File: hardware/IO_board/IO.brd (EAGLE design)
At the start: 167.9 x 122.5 mm, 52 parts, among them IC1 MAX232, IC4 74HCT139N, IC5 74AC06N, IC7 MAX232, J1 DIN5, X2 CRYSTALS-NOGND-CFPX-217

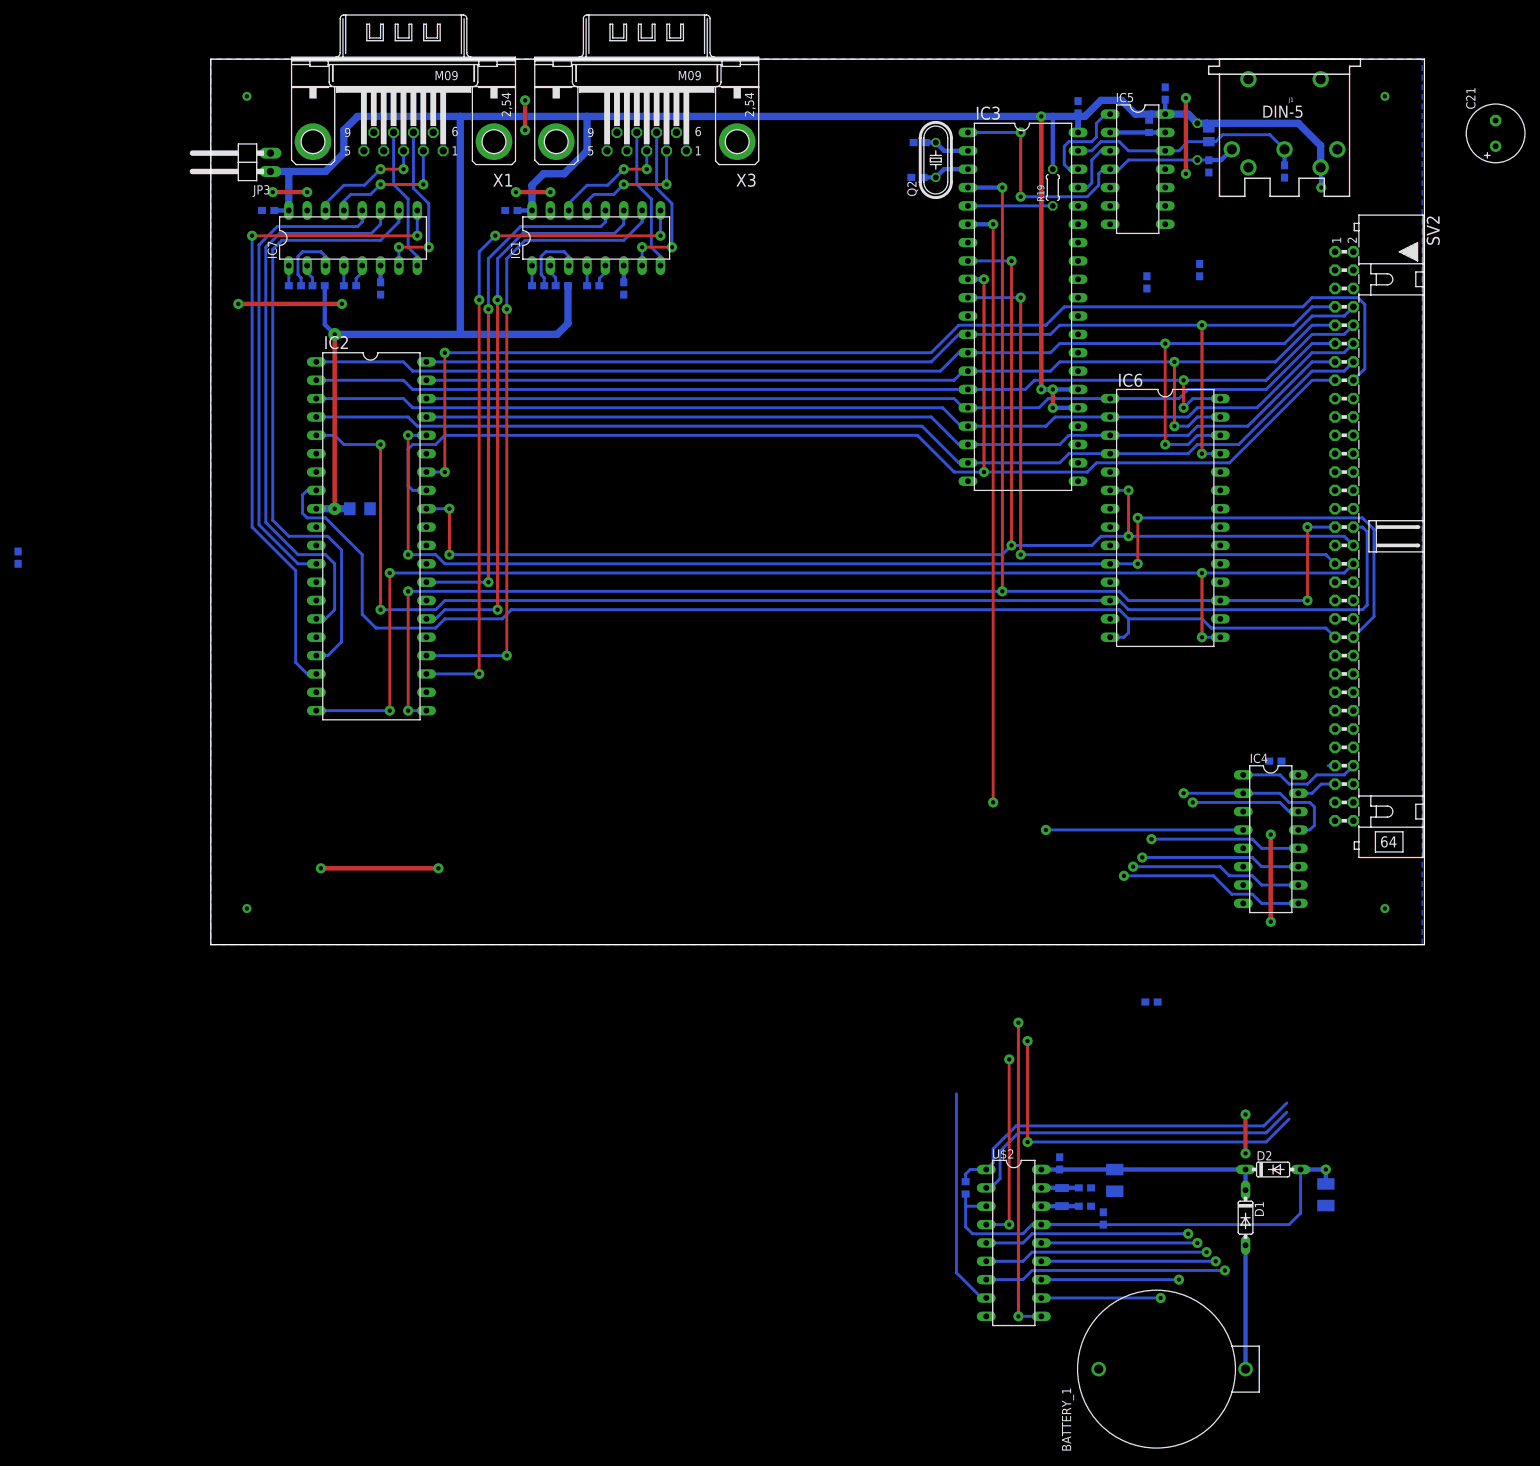
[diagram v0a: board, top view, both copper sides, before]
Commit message: CPU board and I/O board update
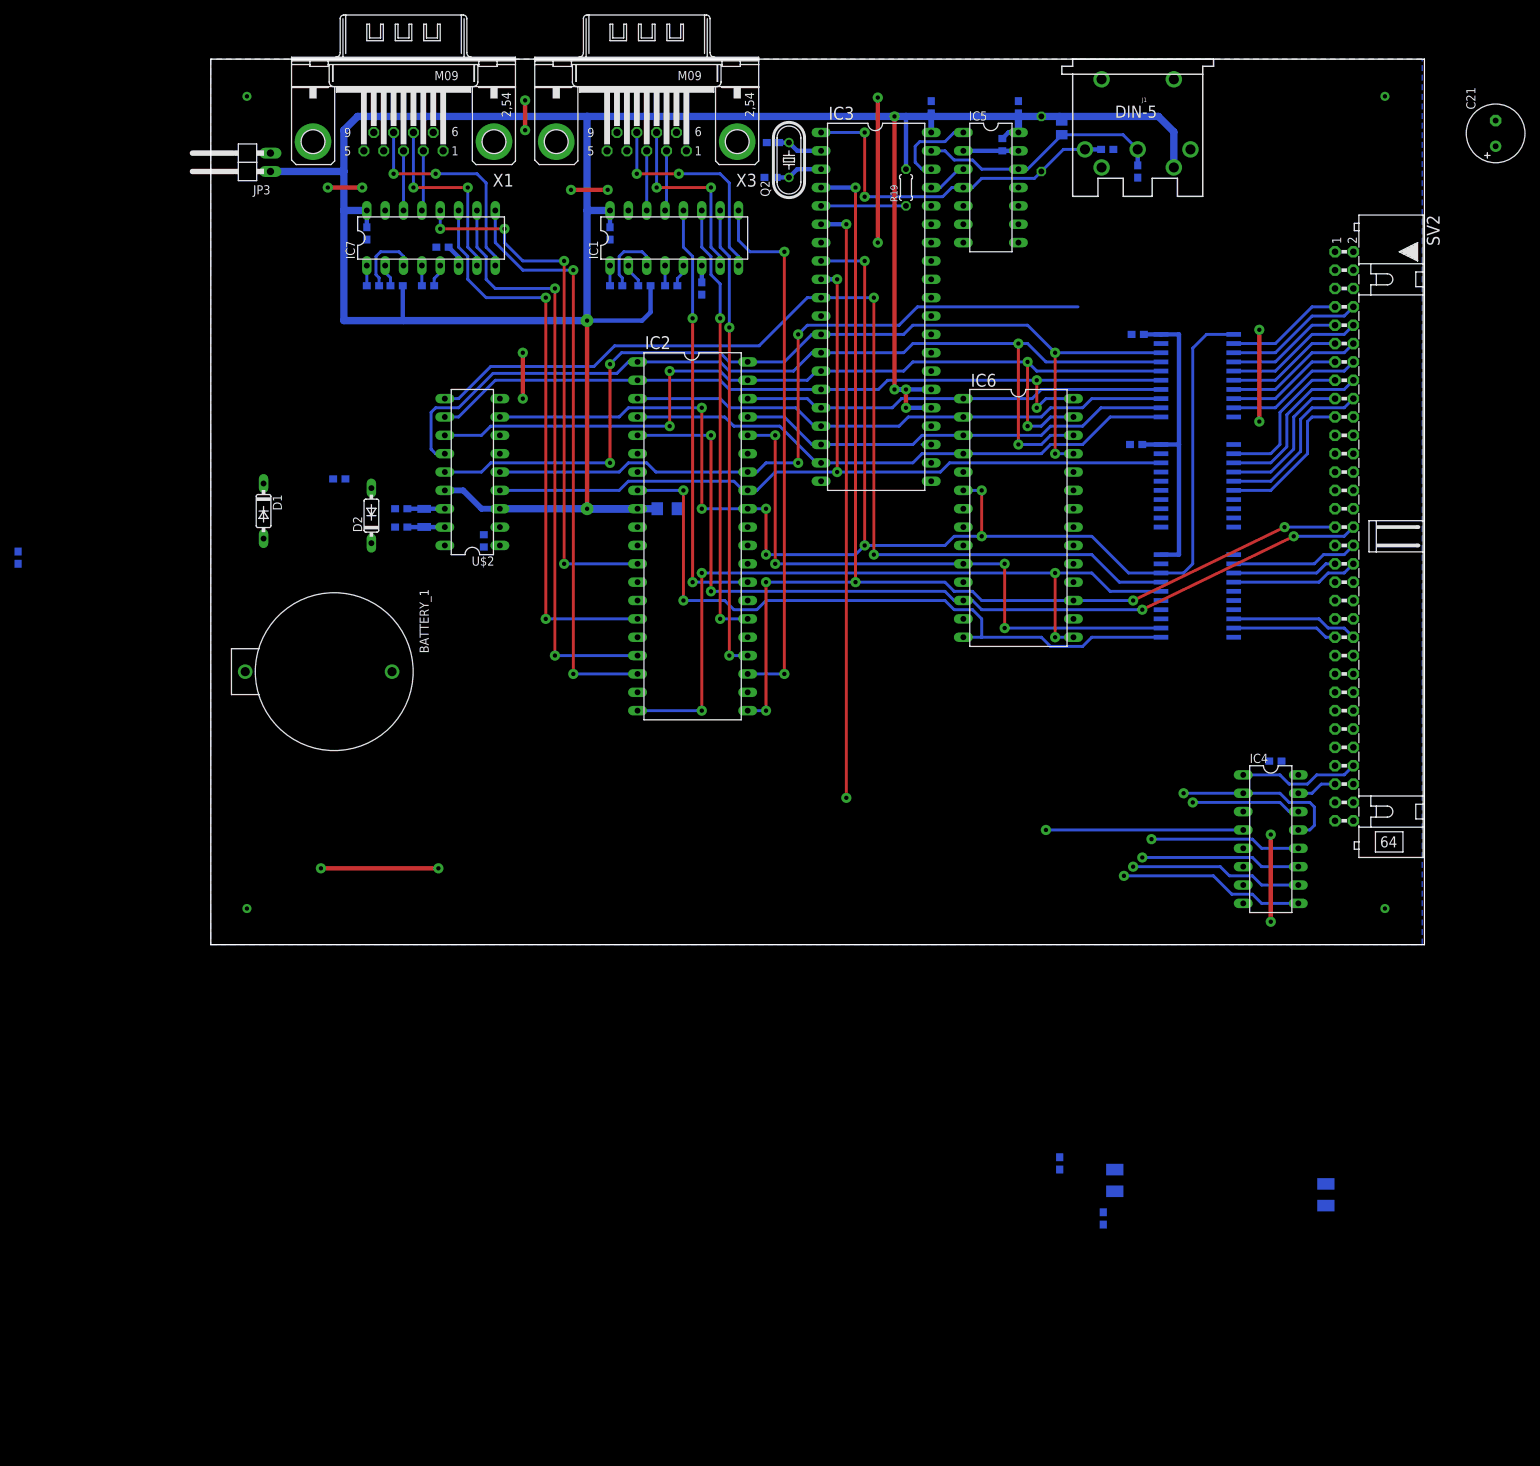
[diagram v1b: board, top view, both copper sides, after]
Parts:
- added IC10, IC8, IC9: 74HCT245DW, 74xx-eu:SO20W
- R7: device rcl:0204/5 -> rcl:0204/7
- moved BATTERY_1 168.8 mm to (4.76, 37.8), turned to 270 degrees
- moved D1 167.4 mm to (7.30, 60.0)
- moved D2 154.1 mm to (22.2, 59.4), turned to 90 degrees
- moved C23 135.2 mm to (26.4, 60.3), turned to 180 degrees
- moved C3 133.7 mm to (17.8, 64.5)
- moved C20 131.6 mm to (26.4, 57.8), turned to 180 degrees
- moved U$2 130.4 mm to (36.2, 65.4), turned to 90 degrees
- moved X2 128.9 mm to (29.5, 59.1), turned to 90 degrees
- moved R10 111.6 mm to (37.8, 55.9), turned to 270 degrees
- moved IC2 44.4 mm to (66.7, 56.5)
- moved C2 42.5 mm to (63.2, 60.3)
- moved C1 22.5 mm to (128.1, 69.2), turned to 0 degrees
- moved R7 21.6 mm to (114.9, 110.8)
- moved IC5 20.5 mm to (108.0, 104.8)
- moved R9 20.5 mm to (109.5, 110.7)
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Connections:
- new net !IORQ_IN: IC9.8, SV2.44
- new net A0_IN: IC10.2, SV2.15
- new net A1_IN: IC10.3, SV2.16
- new net A2_IN: IC10.4, SV2.17
- new net A3_IN: IC10.5, SV2.18
- new net A4_IN: IC10.6, SV2.19
- new net CLK_IN: IC9.4, SV2.36
- new net D0_IN: IC8.2, SV2.7
- new net D1_IN: IC8.3, SV2.8
- new net D2_IN: IC8.4, SV2.9
- new net D3_IN: IC8.5, SV2.10
- new net D4_IN: IC8.6, SV2.11
- new net D5_IN: IC8.7, SV2.12
- new net D6_IN: IC8.8, SV2.13
- new net D7_IN: IC8.9, SV2.14
- new net M1_IN: IC9.9, SV2.43
- new net RD_IN: IC9.2, SV2.34
- new net WR_IN: IC9.3, SV2.35
- net !IORQ: now also IC9.12; no longer SV2.44
- net A0: now also IC10.18; no longer SV2.15
- net A1: now also IC10.17; no longer SV2.16
- net A2: now also IC10.16; no longer SV2.17
- net A3: now also IC10.15; no longer SV2.18
- net A4: now also IC10.14; no longer SV2.19
- net CLK: now also IC9.16; no longer SV2.36
- net D0: now also IC8.18; no longer SV2.7
- net D1: now also IC8.17; no longer SV2.8
- net D2: now also IC8.16; no longer SV2.9
- net D3: now also IC8.15; no longer SV2.10
- net D4: now also IC8.14; no longer SV2.11
- net D5: now also IC8.13; no longer SV2.12
- net D6: now also IC8.12; no longer SV2.13
- net D7: now also IC8.11; no longer SV2.14
- net GND: now also IC10.10, IC10.19, IC10.7, IC10.8, IC10.9, IC8.10, IC8.19, IC9.10, IC9.19, IC9.5, IC9.6, IC9.7
- net M1: now also IC9.11; no longer SV2.43
- net RD: now also IC8.1, IC9.18; no longer SV2.34
- net VCC: now also IC10.20, IC8.20, IC9.20
- net WR: now also IC9.17; no longer SV2.35
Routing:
- net !IORQ: track 176.4 -> 83.9 mm
- net A1: track 189.5 -> 100.9 mm, vias 3 -> 2
- net A0: track 199.2 -> 123.0 mm, vias 4 -> 2
- net D7: track 151.9 -> 77.7 mm
- net D5: track 149.8 -> 75.6 mm
- net D4: track 129.9 -> 58.8 mm
- net D6: track 132.0 -> 60.9 mm
- net CLK: track 174.5 -> 104.0 mm
- net M1: track 166.3 -> 95.9 mm, vias 0 -> 2
- net D3: track 174.3 -> 112.3 mm, vias 3 -> 2
- net INT: track 182.4 -> 124.6 mm, vias 2 -> 4
- net D1: track 194.0 -> 136.4 mm, vias 3 -> 2
- net !RESET: track 218.6 -> 161.8 mm
- net UART_CS: track 72.3 -> 20.8 mm, vias 3 -> 1
- net RTC_IRQ: track 50.7 -> 0.00 mm
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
